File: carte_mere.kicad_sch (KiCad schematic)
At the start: 16 parts, among them J20 Conn_01x02_Pin, J21 Conn_01x02_Pin, J22 Conn_01x02_Pin, J23 Conn_01x02_Pin, J24 Conn_01x02_Pin, U3 R-78B3.3-2.0, U4 R-78B5.0-2.0

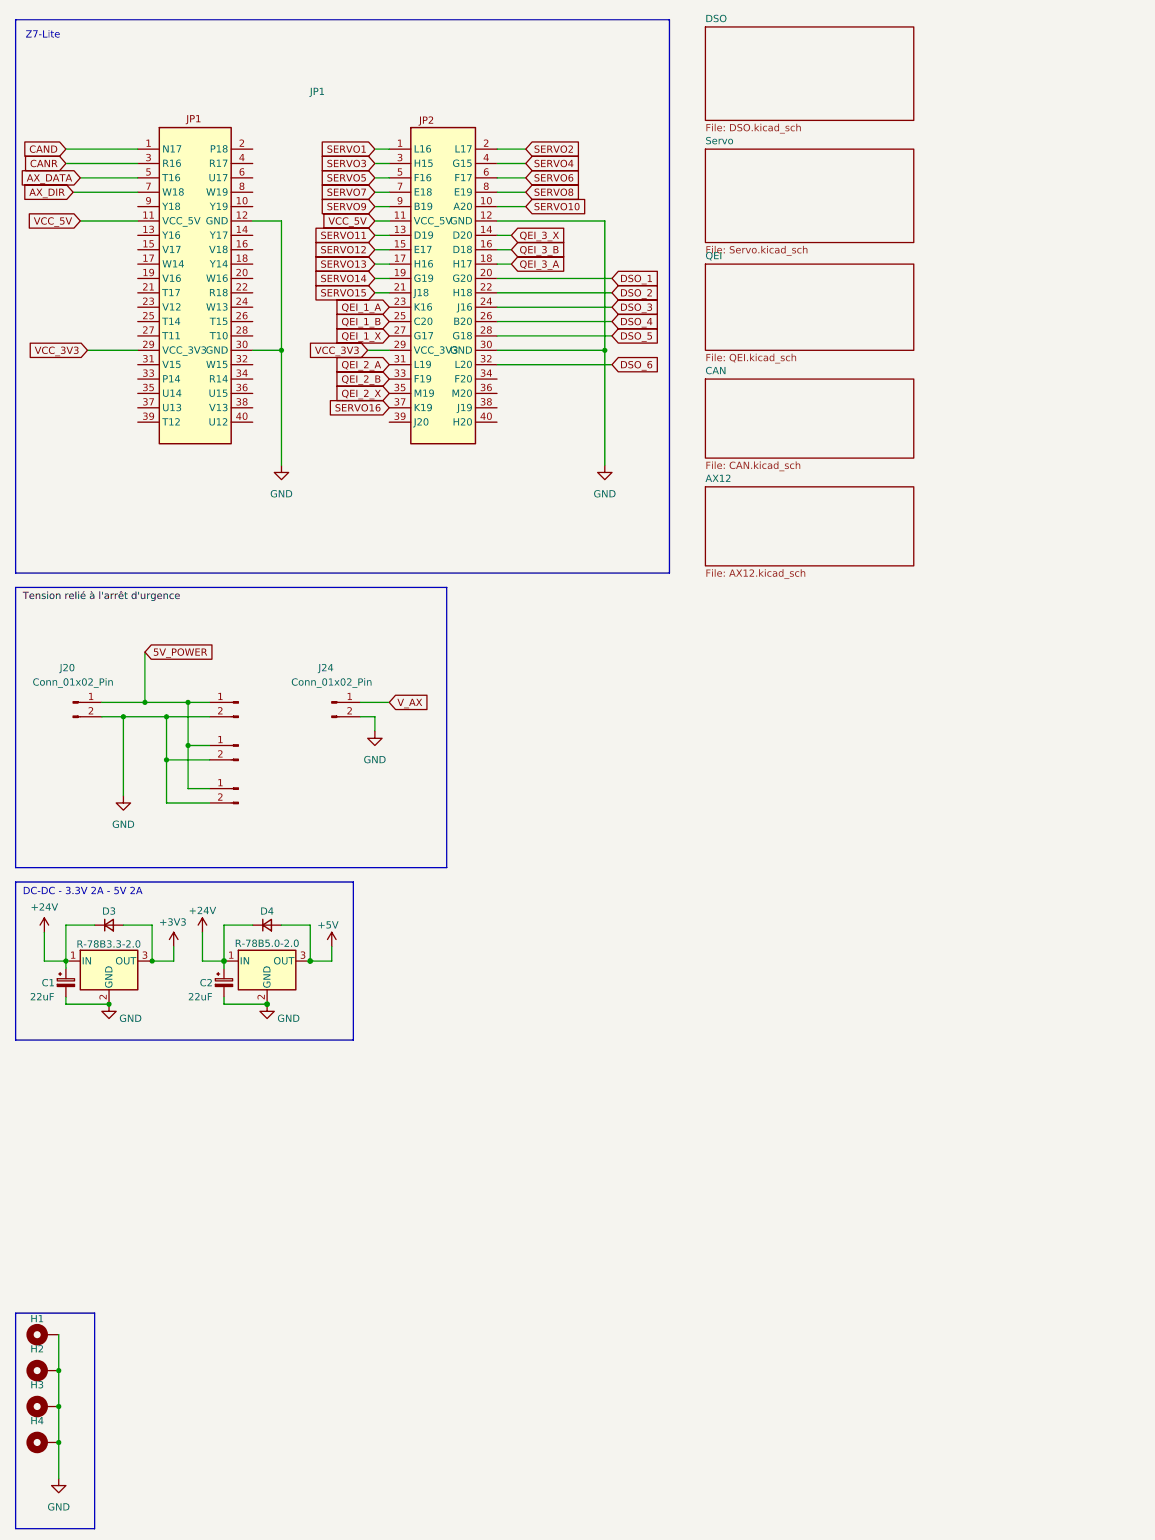
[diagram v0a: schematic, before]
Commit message: update
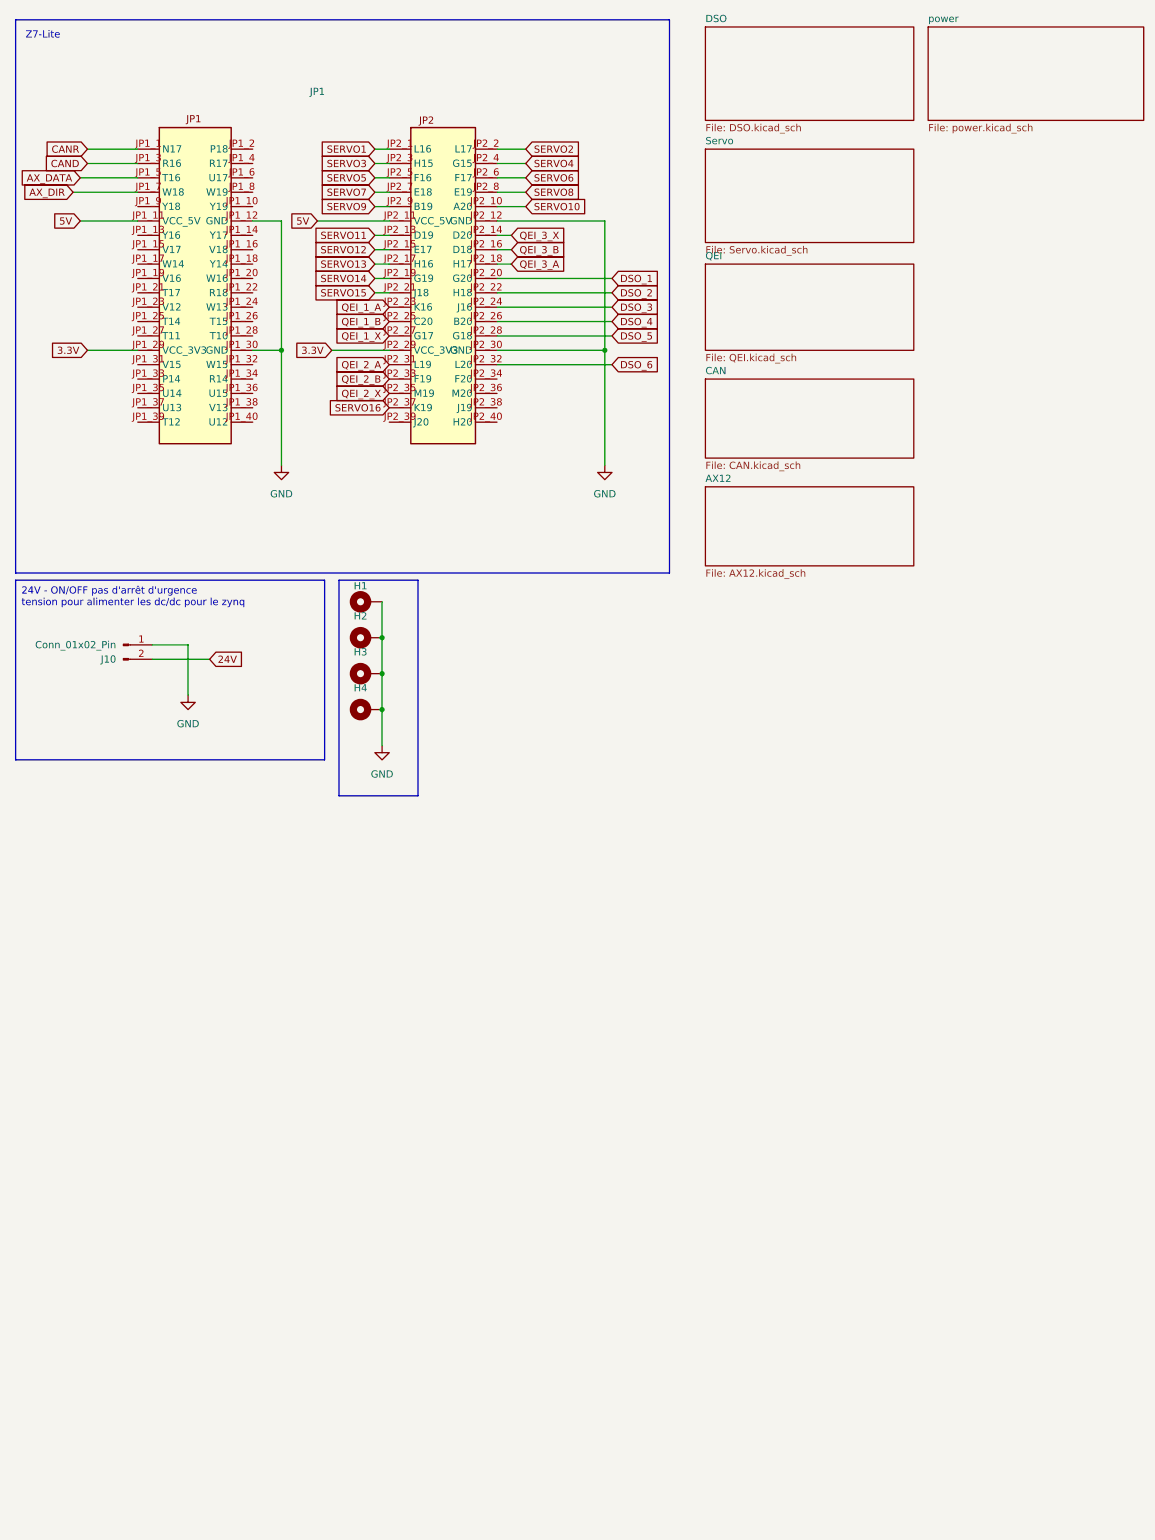
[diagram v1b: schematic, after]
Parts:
- removed C1, C2: 22uF, Capacitor_SMD:CP_Elec_5x5.4, symbol Device:CP_Small
- removed D3, D4: D_Small, Diode_SMD:D_SMA_Handsoldering, symbol Device:D_Small
- removed J20, J21, J22, J23, J24: Conn_01x02_Pin, symbol Connector:Conn_01x02_Pin
- removed U3: R-78B3.3-2.0, Converter_DCDC:Converter_DCDC_RECOM_R-78B-2.0_THT, symbol Regulator_Switching:R-78B3.3-2.0
- removed U4: R-78B5.0-2.0, Converter_DCDC:Converter_DCDC_RECOM_R-78B-2.0_THT, symbol Regulator_Switching:R-78B5.0-2.0
- added J10: Conn_01x02_Pin, Connector_AMASS:AMASS_XT30U-F_1x02_P5.0mm_Vertical, symbol Connector:Conn_01x02_Pin
- JP1: footprint (none) -> Z7-lite:Z7-lite
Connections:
- net AX_DATA: now also JP1.JP1_5 (T16); no longer JP1.5 (T16)
- net AX_DIR: now also JP1.JP1_7 (W18); no longer JP1.7 (W18)
- net CAND: now also JP1.JP1_3 (R16); no longer JP1.1 (N17)
- net CANR: now also JP1.JP1_1 (N17); no longer JP1.3 (R16)
- net DSO_1: now also JP1.JP2_20 (G20); no longer JP1.20 (W16)
- net DSO_2: now also JP1.JP2_22 (H18); no longer JP1.22 (R18)
- net DSO_3: now also JP1.JP2_24 (J16); no longer JP1.24 (W13)
- net DSO_4: now also JP1.JP2_26 (B20); no longer JP1.26 (T15)
- net DSO_5: now also JP1.JP2_28 (G18); no longer JP1.28 (T10)
- net DSO_6: now also JP1.JP2_32 (L20); no longer JP1.32 (W15)
- net GND: now also JP1.JP1_12 (GND), JP1.JP1_30 (GND), JP1.JP2_12 (GND), JP1.JP2_30 (GND), J10.1 (Pin_1); no longer JP1.12 (GND), JP1.30 (GND)
- net QEI_1_A: now also JP1.JP2_23 (K16); no longer JP1.23 (V12)
- net QEI_1_B: now also JP1.JP2_25 (C20); no longer JP1.25 (T14)
- net QEI_1_X: now also JP1.JP2_27 (G17); no longer JP1.27 (T11)
- net QEI_2_A: now also JP1.JP2_31 (L19); no longer JP1.31 (V15)
- net QEI_2_B: now also JP1.JP2_33 (F19); no longer JP1.33 (P14)
- net QEI_2_X: now also JP1.JP2_35 (M19); no longer JP1.35 (U14)
- net QEI_3_A: now also JP1.JP2_18 (H17); no longer JP1.18 (Y14)
- net QEI_3_B: now also JP1.JP2_16 (D18); no longer JP1.16 (V18)
- net QEI_3_X: now also JP1.JP2_14 (D20); no longer JP1.14 (Y17)
- net SERVO1: now also JP1.JP2_1 (L16); no longer JP1.1 (N17)
- net SERVO10: now also JP1.JP2_10 (A20); no longer JP1.10 (Y19)
- net SERVO11: now also JP1.JP2_13 (D19); no longer JP1.13 (Y16)
- net SERVO12: now also JP1.JP2_15 (E17); no longer JP1.15 (V17)
- net SERVO13: now also JP1.JP2_17 (H16); no longer JP1.17 (W14)
- net SERVO14: now also JP1.JP2_19 (G19); no longer JP1.19 (V16)
- net SERVO15: now also JP1.JP2_21 (J18); no longer JP1.21 (T17)
- net SERVO16: now also JP1.JP2_37 (K19); no longer JP1.37 (U13)
- net SERVO2: now also JP1.JP2_2 (L17); no longer JP1.2 (P18)
- net SERVO3: now also JP1.JP2_3 (H15); no longer JP1.3 (R16)
- net SERVO4: now also JP1.JP2_4 (G15); no longer JP1.4 (R17)
- net SERVO5: now also JP1.JP2_5 (F16); no longer JP1.5 (T16)
- net SERVO6: now also JP1.JP2_6 (F17); no longer JP1.6 (U17)
- net SERVO7: now also JP1.JP2_7 (E18); no longer JP1.7 (W18)
- net SERVO8: now also JP1.JP2_8 (E19); no longer JP1.8 (W19)
- net SERVO9: now also JP1.JP2_9 (B19); no longer JP1.9 (Y18)
- removed net VCC_3V3: JP1.29 (VCC_3V3)
- removed net VCC_5V: JP1.11 (VCC_5V)
- new net 24V: J10.2 (Pin_2)
- new net 3.3V: JP1.JP1_29 (VCC_3V3), JP1.JP2_29 (VCC_3V3)
- new net 5V: JP1.JP1_11 (VCC_5V), JP1.JP2_11 (VCC_5V)
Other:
- added sheet power (power.kicad_sch)
- note removed: "DC-DC - 3.3V 2A - 5V 2A"
- moved on the sheet: H1, H2, H3, H4

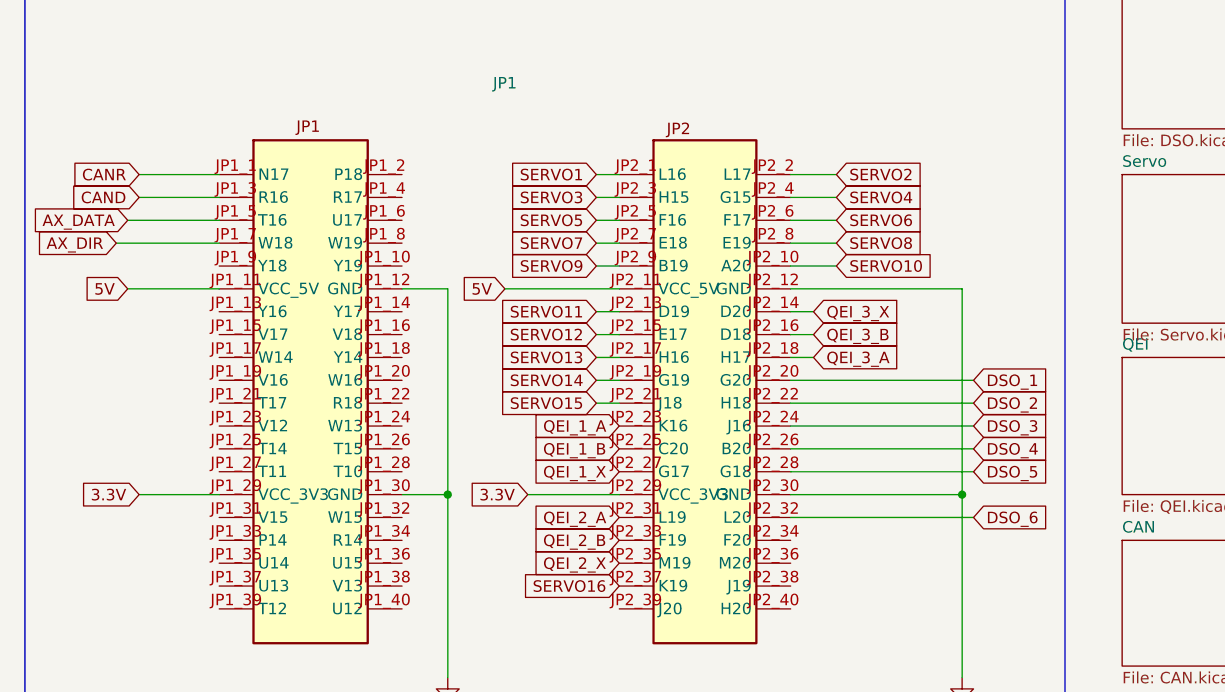
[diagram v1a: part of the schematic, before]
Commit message: update schematic + layout
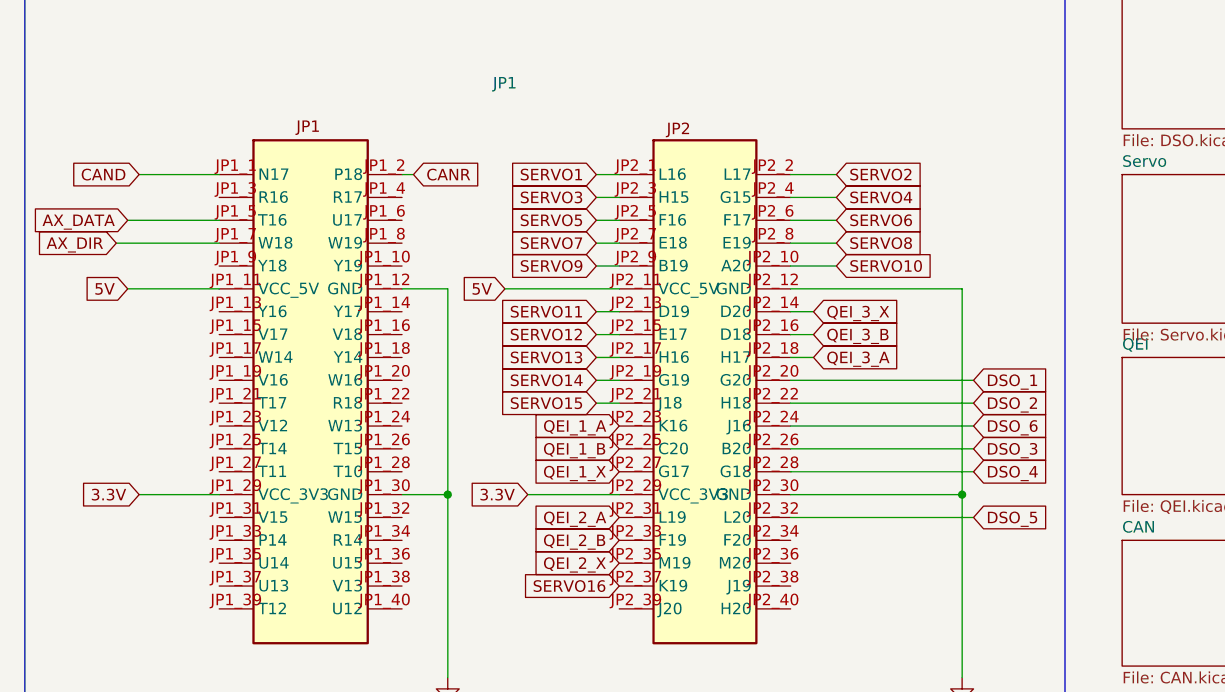
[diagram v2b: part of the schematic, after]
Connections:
- net CAND: now also JP1.JP1_1 (N17); no longer JP1.JP1_3 (R16)
- net CANR: now also JP1.JP1_2 (P18); no longer JP1.JP1_1 (N17)
- net DSO_3: now also JP1.JP2_26 (B20); no longer JP1.JP2_24 (J16)
- net DSO_4: now also JP1.JP2_28 (G18); no longer JP1.JP2_26 (B20)
- net DSO_5: now also JP1.JP2_32 (L20); no longer JP1.JP2_28 (G18)
- net DSO_6: now also JP1.JP2_24 (J16); no longer JP1.JP2_32 (L20)
